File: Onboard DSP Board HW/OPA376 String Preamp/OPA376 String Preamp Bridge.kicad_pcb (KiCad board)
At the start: 2 copper layers, 28.4 x 92.7 mm, 49 parts, among them J1 Input, J10 Input, J14 Input, J5 Input, U1 OPA376AIDCKT, U2 OPA376AIDCKT, U3 OPA376AIDCKT, U4 OPA376AIDCKT

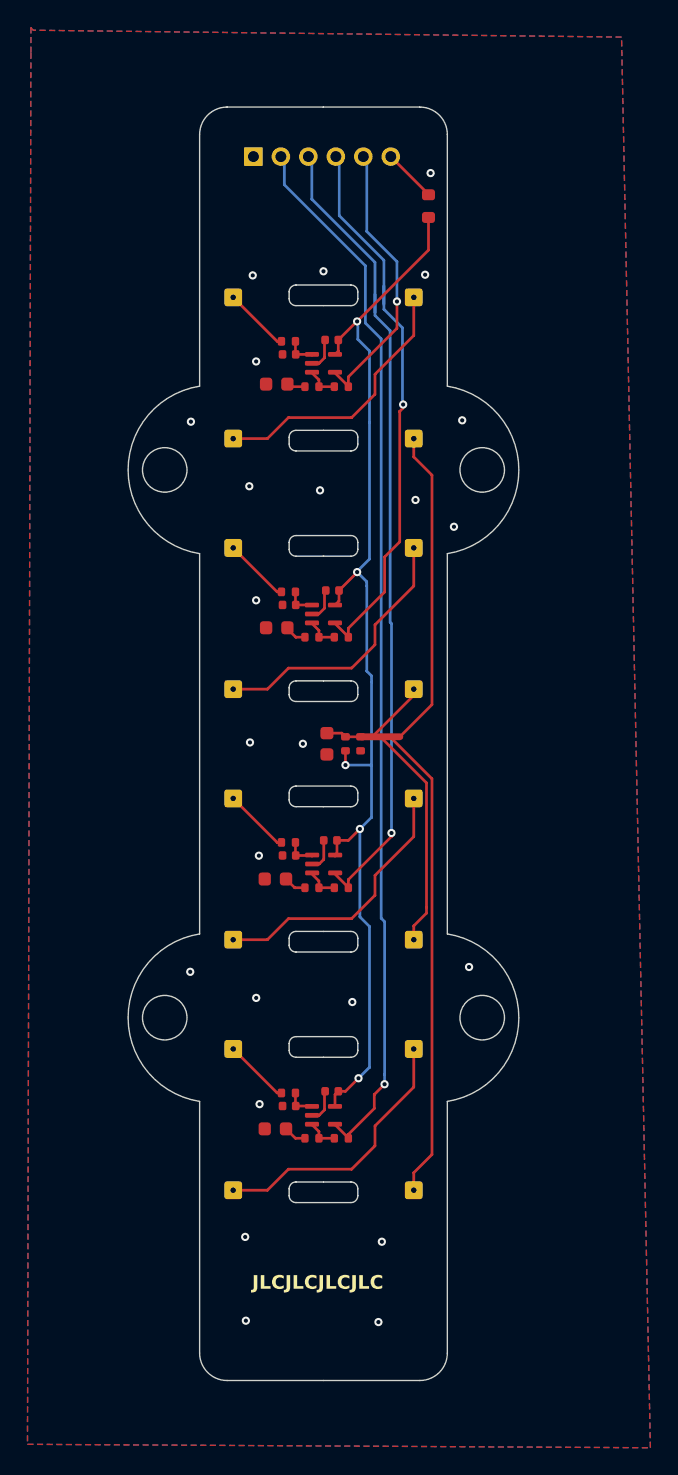
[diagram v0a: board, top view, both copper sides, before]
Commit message: WIP
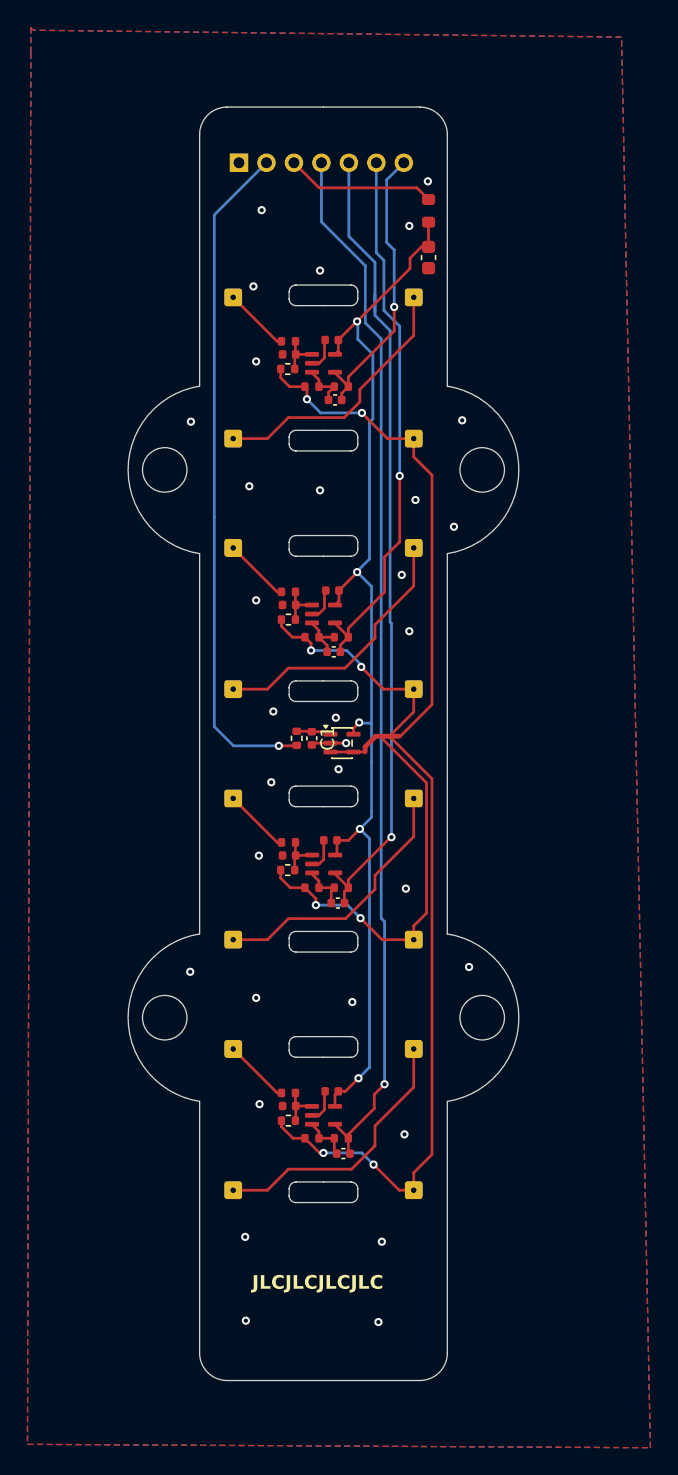
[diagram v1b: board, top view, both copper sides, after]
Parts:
- removed C2: 10uF, Capacitor_SMD:C_0603_1608Metric
- removed J9: ~, Connector_PinHeader_2.00mm:PinHeader_1x06_P2.00mm_Horizontal
- removed R1: 100K, Resistor_SMD:R_0402_1005Metric
- added C21: 220pF, Capacitor_SMD:C_0402_1005Metric, F.Cu at (101.4, 129.8)
- added C3: 100nF, Capacitor_SMD:C_0603_1608Metric, F.Cu at (107.7, 64.6)
- added J18: ~, Connector_PinHeader_2.00mm:PinHeader_1x07_P2.00mm_Horizontal, B.Cu at (93.8, 57.7)
- added R25: 27K, Resistor_SMD:R_0402_1005Metric, F.Cu at (97.4, 72.7)
- added R26: 27K, Resistor_SMD:R_0402_1005Metric, F.Cu at (97.4, 91.0)
- added R27: 27K, Resistor_SMD:R_0402_1005Metric, F.Cu at (97.4, 109.2)
- added R28: 27K, Resistor_SMD:R_0402_1005Metric, F.Cu at (97.4, 127.4)
- added U5: OPA376AIDCKR, Package_TO_SOT_SMD:SOT-353_SC-70-5, F.Cu at (101.3, 100.0)
- C1: value 22uF -> 100pF; footprint Capacitor_SMD:C_0603_1608Metric -> Capacitor_SMD:C_0402_1005Metric
- C11, C13, C15: value 22uF -> 220pF; footprint Capacitor_SMD:C_0603_1608Metric -> Capacitor_SMD:C_0402_1005Metric
- R2: value 43K -> 1K
- U1, U2, U3, U4: value OPA376AIDCKT -> OPA376AIDCKR
- moved C1 25.9 mm to (99.2, 99.6), turned to -90 degrees
- moved C11 17.1 mm to (100.8, 75.0), turned to 180 degrees
- moved C13 17.1 mm to (100.7, 93.3), turned to 180 degrees
- moved C15 17.1 mm to (101.0, 111.6), turned to 180 degrees
- moved R2 4.67 mm to (98.0, 99.6), turned to 90 degrees
- moved R3 0.35 mm to (107.7, 61.2), turned to -90 degrees
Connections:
- net /Input renamed /SIngle FET preamp/in
- net /SIngle FET preamp1/Input renamed /SIngle FET preamp1/in
- net /SIngle FET preamp2/Input renamed /SIngle FET preamp2/in
- net /SIngle FET preamp3/Input renamed /SIngle FET preamp3/in
- C1 pad 1: GND -> Net-(U5-+)
- C1 pad 2: Net-(C1-Pad2) -> GND
- C11 pad 1: GND -> /SIngle FET preamp/Output
- C11 pad 2: Net-(C11-Pad2) -> Net-(U1--)
- C13 pad 1: GND -> /SIngle FET preamp1/Output
- C13 pad 2: Net-(C13-Pad2) -> Net-(U2--)
- C15 pad 1: GND -> /SIngle FET preamp2/Output
- C15 pad 2: Net-(C15-Pad2) -> Net-(U3--)
- R14 pad 1: Net-(C1-Pad2) -> /SIngle FET preamp/MidRail
- R17 pad 1: Net-(C11-Pad2) -> /SIngle FET preamp/MidRail
- R2 pad 1: /SIngle FET preamp/MidRail -> /Bias
- R2 pad 2: GND -> Net-(U5-+)
- R20 pad 1: Net-(C13-Pad2) -> /SIngle FET preamp/MidRail
- R23 pad 1: Net-(C15-Pad2) -> /SIngle FET preamp/MidRail
- R3 pad 1: /SIngle FET preamp/3.3V -> /3V3
- R3 pad 2: Net-(J9-Pin_6) -> /SIngle FET preamp/3.3V
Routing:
- net /SIngle FET preamp/MidRail: track 85.6 -> 135.1 mm, vias 0 -> 8
- net /Bias: track 0.00 -> 49.2 mm, vias 0 -> 1
- net /3V3: track 0.00 -> 10.9 mm
- net Net-(J9-Pin_6): track 4.07 -> 0.00 mm
- net GND: track 9.63 -> 12.4 mm, vias 24 -> 32
- net Net-(U5-+): track 0.00 -> 2.55 mm
- net /SIngle FET preamp1/Output: track 41.4 -> 39.5 mm
- net Net-(C15-Pad2): track 1.70 -> 0.00 mm
- net Net-(C13-Pad2): track 1.68 -> 0.00 mm
- net Net-(C11-Pad2): track 1.62 -> 0.00 mm
- net Net-(C1-Pad2): track 1.40 -> 0.00 mm
- net Net-(U2--): track 2.33 -> 3.64 mm
- net Net-(U3--): track 2.33 -> 3.54 mm
- net Net-(U4--): track 2.33 -> 3.52 mm
- net Net-(U1--): track 2.33 -> 3.47 mm
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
